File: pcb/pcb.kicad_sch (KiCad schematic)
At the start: 113 parts, among them J1 MJ-4PP-9, J2 MJ-4PP-9, J3 USB_C_Receptacle_USB2.0_16P, J4 USB to TTL, J5 Conn_01x03, J6 Conn_01x03, SW1 KEY_SW, SW10 KEY_SW, SW11 KEY_SW, SW12 KEY_SW, SW13 KEY_SW, SW14 KEY_SW, SW15 KEY_SW, SW16 KEY_SW, SW17 KEY_SW, SW18 KEY_SW, SW19 KEY_SW, SW2 KEY_SW, SW20 KEY_SW, SW21 KEY_SW, SW22 KEY_SW, SW23 KEY_SW, SW24 KEY_SW, SW25 KEY_SW, SW26 KEY_SW, SW27 RotaryEncoder, SW3 KEY_SW, SW30 KEY_SW, SW31 KEY_SW, SW32 KEY_SW, SW33 KEY_SW, SW34 KEY_SW, SW35 KEY_SW, SW36 KEY_SW, SW37 KEY_SW, SW38 KEY_SW, SW39 KEY_SW, SW4 KEY_SW, SW40 KEY_SW, SW41 KEY_SW, SW42 KEY_SW, SW43 KEY_SW, SW44 KEY_SW, SW45 KEY_SW, SW46 KEY_SW, SW47 KEY_SW, SW48 KEY_SW, SW49 KEY_SW, SW5 KEY_SW, SW50 KEY_SW, SW51 KEY_SW, SW52 KEY_SW, SW53 KEY_SW, SW54 KEY_SW, SW6 KEY_SW, SW60 RESET_SW, SW61 BOOT_SW, SW7 KEY_SW, SW8 KEY_SW, SW9 KEY_SW, SW６２1 DIP_SW, U1 ESP32-S3-WROOM-1, U2 TPS1117LV33S, U3 USBLC6-2SC6

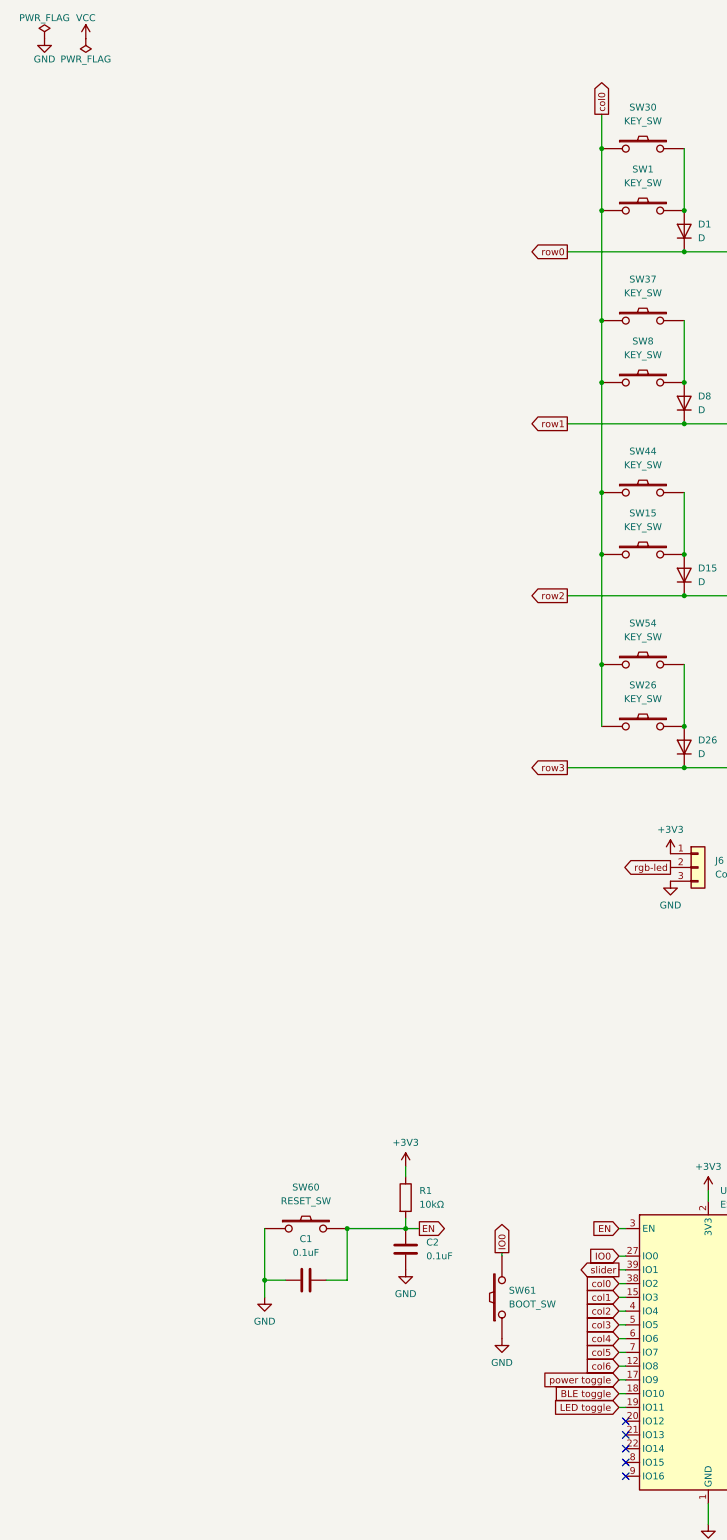
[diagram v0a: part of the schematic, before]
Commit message: connect
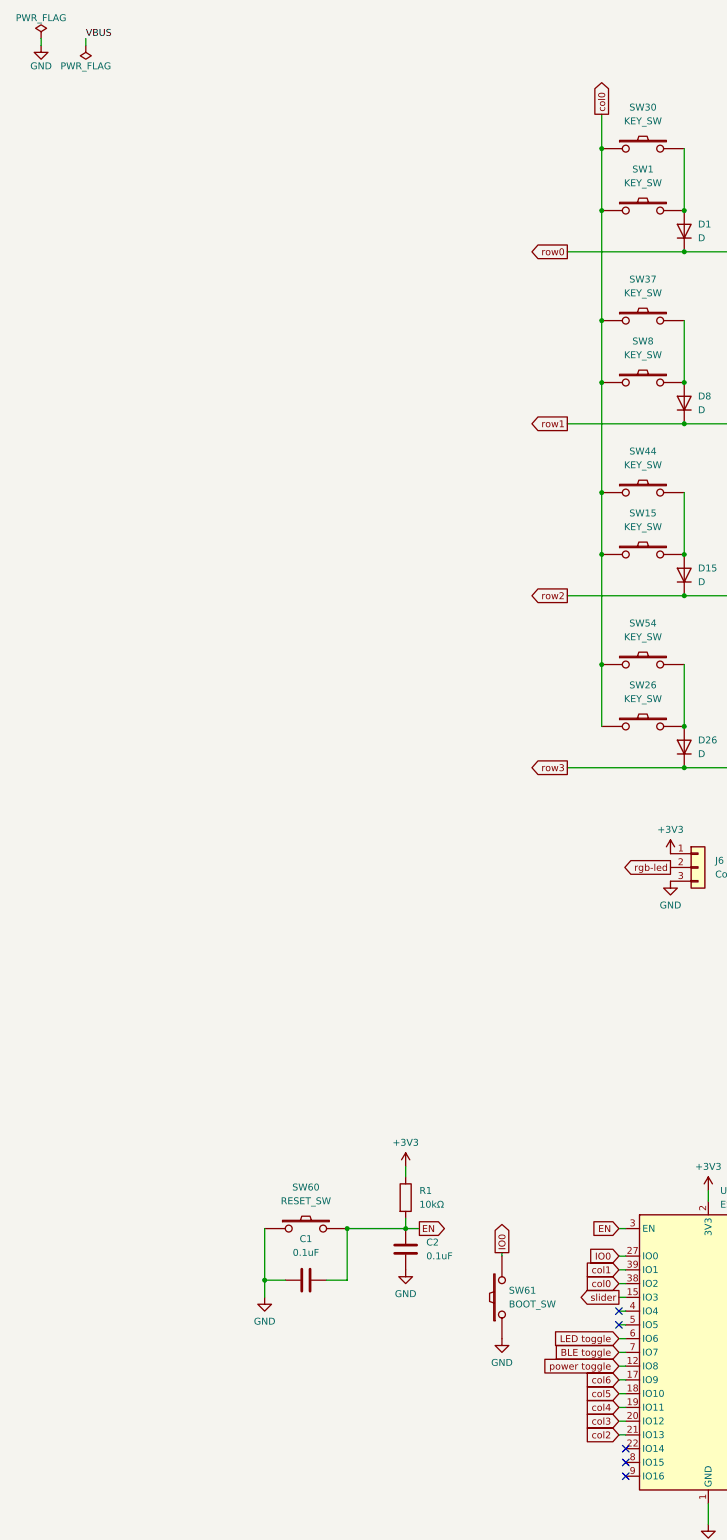
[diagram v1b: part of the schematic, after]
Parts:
- J3: footprint Connector_USB:USB_C_Receptacle_GCT_USB4105-xx-A_16P_TopMnt_Horizontal -> lib:USB_C_Receptacle_GCT_USB4105-xx-A_16P_TopMnt_Horizontal_rev
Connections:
- net BLE toggle: now also U1.7 (IO7); no longer U1.18 (IO10)
- net LED toggle: now also U1.6 (IO6); no longer U1.19 (IO11)
- net col1: now also U1.39 (IO1); no longer U1.15 (IO3)
- net col2: now also U1.21 (IO13); no longer U1.4 (IO4)
- net col3: now also U1.20 (IO12); no longer U1.5 (IO5)
- net col4: now also U1.19 (IO11); no longer U1.6 (IO6)
- net col5: now also U1.18 (IO10); no longer U1.7 (IO7)
- net col6: now also U1.17 (IO9); no longer U1.12 (IO8)
- net power toggle: now also U1.12 (IO8); no longer U1.17 (IO9)
- net slider: now also U1.15 (IO3); no longer U1.39 (IO1)
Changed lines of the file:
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@@
 	)
 	(no_connect
-		(at 142.875 240.03)
+		(at 111.125 242.57)
 	)
 	(no_connect
-		(at 112.395 260.35)
+		(at 142.875 240.03)
 	)
 	(no_connect
@@
 	)
 	(no_connect
-		(at 112.395 262.89)
+		(at 112.395 270.51)
 	)
 	(no_connect
-		(at 112.395 270.51)
+		(at 111.125 240.03)
 	)
 	(no_connect
@@
 	(wire
 		(pts
+			(xy 111.125 260.35) (xy 112.395 260.35)
+		)
+		(stroke
+			(width 0)
+			(type default)
+		)
+	)
+	(wire
+		(pts
 			(xy 254 186.055) (xy 254 187.325)
 		)
@@
 	(wire
 		(pts
+			(xy 12.7 6.35) (xy 12.7 5.08)
+		)
+		(stroke
+			(width 0)
+			(type default)
+		)
+	)
+	(wire
+		(pts
 			(xy 60.96 234.315) (xy 57.15 234.315)
 		)
@@
 	(wire
 		(pts
+			(xy 111.125 262.89) (xy 112.395 262.89)
+		)
+		(stroke
+			(width 0)
+			(type default)
+		)
+	)
+	(wire
+		(pts
 			(xy 233.68 149.225) (xy 233.68 150.495)
 		)
@@
 	(wire
 		(pts
+			(xy 4.445 6.35) (xy 4.445 5.08)
+		)
+		(stroke
+			(width 0)
+			(type default)
+		)
+	)
+	(wire
+		(pts
 			(xy 176.53 254) (xy 177.8 254)
 		)
@@
 		)
 	)
+	(label "VBUS"
+		(at 12.7 5.08 0)
+		(fields_autoplaced yes)
+		(effects
+			(font
+				(size 1.27 1.27)
+			)
+			(justify left bottom)
+		)
+	)
 	(global_label "col5"
 		(shape output)
@@
 	(global_label "LED toggle"
 		(shape input)
-		(at 111.125 257.81 180)
+		(at 111.125 245.11 180)
 		(fields_autoplaced yes)
 		(effects
@@
 		)
 		(property "Intersheetrefs" "${INTERSHEET_REFS}"
-			(at 97.7986 257.81 0)
+			(at 97.7986 245.11 0)
 			(effects
 				(font
@@
 	(global_label "col6"
 		(shape input)
-		(at 111.125 250.19 180)
+		(at 111.125 252.73 180)
 		(fields_autoplaced yes)
 		(effects
@@
 		)
 		(property "Intersheetrefs" "${INTERSHEET_REFS}"
-			(at 104.0275 250.19 0)
+			(at 104.0275 252.73 0)
 			(effects
 				(font
@@
 	(global_label "BLE toggle"
 		(shape input)
-		(at 111.125 255.27 180)
+		(at 111.125 247.65 180)
 		(fields_autoplaced yes)
 		(effects
@@
 		)
 		(property "Intersheetrefs" "${INTERSHEET_REFS}"
-			(at 97.7986 255.27 0)
+			(at 97.7986 247.65 0)
 			(effects
 				(font
@@
 	(global_label "power toggle"
 		(shape input)
-		(at 111.125 252.73 180)
+		(at 111.125 250.19 180)
 		(fields_autoplaced yes)
 		(effects
@@
 		)
 		(property "Intersheetrefs" "${INTERSHEET_REFS}"
-			(at 95.7424 252.73 0)
+			(at 95.7424 250.19 0)
 			(effects
 				(font
@@
 	(global_label "col2"
 		(shape input)
-		(at 111.125 240.03 180)
+		(at 111.125 262.89 180)
 		(fields_autoplaced yes)
 		(effects
@@
 		)
 		(property "Intersheetrefs" "${INTERSHEET_REFS}"
-			(at 104.0275 240.03 0)
+			(at 104.0275 262.89 0)
 			(effects
 				(font
@@
 	(global_label "col3"
 		(shape input)
-		(at 111.125 242.57 180)
+		(at 111.125 260.35 180)
 		(fields_autoplaced yes)
 		(effects
@@
 		)
 		(property "Intersheetrefs" "${INTERSHEET_REFS}"
-			(at 104.0275 242.57 0)
+			(at 104.0275 260.35 0)
 			(effects
 				(font
@@
 	(global_label "col5"
 		(shape input)
-		(at 111.125 247.65 180)
+		(at 111.125 255.27 180)
 		(fields_autoplaced yes)
 		(effects
@@
 		)
 		(property "Intersheetrefs" "${INTERSHEET_REFS}"
-			(at 104.0275 247.65 0)
+			(at 104.0275 255.27 0)
 			(effects
 				(font
@@
 	(global_label "col1"
 		(shape input)
-		(at 111.125 237.49 180)
+		(at 111.125 232.41 180)
 		(fields_autoplaced yes)
 		(effects
@@
 		)
 		(property "Intersheetrefs" "${INTERSHEET_REFS}"
-			(at 104.0275 237.49 0)
+			(at 104.0275 232.41 0)
 			(effects
 				(font
@@
 	(global_label "col4"
 		(shape input)
-		(at 111.125 245.11 180)
+		(at 111.125 257.81 180)
 		(fields_autoplaced yes)
 		(effects
@@
 		)
 		(property "Intersheetrefs" "${INTERSHEET_REFS}"
-			(at 104.0275 245.11 0)
+			(at 104.0275 257.81 0)
 			(effects
 				(font
@@
 	(global_label "slider"
 		(shape output)
-		(at 111.125 232.41 180)
+		(at 111.125 237.49 180)
 		(fields_autoplaced yes)
 		(effects
@@
 		)
 		(property "Intersheetrefs" "${INTERSHEET_REFS}"
-			(at 102.8179 232.41 0)
+			(at 102.8179 237.49 0)
 			(effects
 				(font
@@
 	)
 	(symbol
-		(lib_id "power:VCC")
-		(at 12.7 5.08 0)
-		(unit 1)
-		(exclude_from_sim no)
-		(in_bom yes)
-		(on_board yes)
-		(dnp no)
-		(property "Reference" "#PWR05"
-			(at 12.7 8.89 0)
-			(effects
-				(font
-					(size 1.27 1.27)
-				)
-				(hide yes)
-			)
-		)
-		(property "Value" "VCC"
-			(at 12.7 1.27 0)
-			(effects
-				(font
-					(size 1.27 1.27)
-				)
-			)
-		)
-		(property "Footprint" ""
-			(at 12.7 5.08 0)
-			(effects
-				(font
-					(size 1.27 1.27)
-				)
-				(hide yes)
-			)
-		)
-		(property "Datasheet" ""
-			(at 12.7 5.08 0)
-			(effects
-				(font
-					(size 1.27 1.27)
-				)
-				(hide yes)
-			)
-		)
-		(property "Description" ""
-			(at 12.7 5.08 0)
-			(effects
-				(font
-					(size 1.27 1.27)
-				)
-				(hide yes)
-			)
-		)
-		(pin "1"
-		)
-		(instances
-			(project "pcb"
-				(path "/ca1682eb-af97-4baf-a70b-d30c3b256c66"
-					(reference "#PWR05")
-					(unit 1)
-				)
-			)
-		)
-	)
-	(symbol
 		(lib_id "Device:D")
 		(at 173.99 104.14 90)
@@
 			)
 		)
-		(property "Footprint" "Connector_USB:USB_C_Receptacle_GCT_USB4105-xx-A_16P_TopMnt_Horizontal"
+		(property "Footprint" "lib:USB_C_Receptacle_GCT_USB4105-xx-A_16P_TopMnt_Horizontal_rev"
 			(at 207.645 234.95 0)
 			(effects
@@
 	(symbol
 		(lib_id "power:PWR_FLAG")
-		(at 5.08 5.08 0)
+		(at 4.445 5.08 0)
 		(unit 1)
 		(exclude_from_sim no)
@@
 		(dnp no)
 		(property "Reference" "#FLG01"
-			(at 5.08 3.175 0)
+			(at 4.445 3.175 0)
 			(effects
 				(font
@@
 		)
 		(property "Value" "PWR_FLAG"
-			(at 5.08 1.27 0)
+			(at 4.445 1.27 0)
 			(effects
 				(font
@@
 		)
 		(property "Footprint" ""
-			(at 5.08 5.08 0)
+			(at 4.445 5.08 0)
 			(effects
 				(font
@@
 		)
 		(property "Datasheet" "~"
-			(at 5.08 5.08 0)
+			(at 4.445 5.08 0)
 			(effects
 				(font
@@
 		)
 		(property "Description" ""
-			(at 5.08 5.08 0)
+			(at 4.445 5.08 0)
 			(effects
 				(font
@@
 	(symbol
 		(lib_id "power:GND")
-		(at 5.08 5.08 0)
+		(at 4.445 6.35 0)
 		(unit 1)
 		(exclude_from_sim no)
@@
 		(dnp no)
 		(property "Reference" "#PWR04"
-			(at 5.08 11.43 0)
+			(at 4.445 12.7 0)
 			(effects
 				(font
@@
 		)
 		(property "Value" "GND"
-			(at 5.08 8.89 0)
+			(at 4.445 10.16 0)
 			(effects
 				(font
@@
 		)
 		(property "Footprint" ""
-			(at 5.08 5.08 0)
+			(at 4.445 6.35 0)
 			(effects
 				(font
@@
 		)
 		(property "Datasheet" ""
-			(at 5.08 5.08 0)
+			(at 4.445 6.35 0)
 			(effects
 				(font
@@
 		)
 		(property "Description" ""
-			(at 5.08 5.08 0)
+			(at 4.445 6.35 0)
 			(effects
 				(font
@@
 	(symbol
 		(lib_id "power:PWR_FLAG")
-		(at 12.7 5.08 180)
+		(at 12.7 6.35 180)
 		(unit 1)
 		(exclude_from_sim no)
@@
 		(dnp no)
 		(property "Reference" "#FLG02"
-			(at 12.7 6.985 0)
+			(at 12.7 8.255 0)
 			(effects
 				(font
@@
 		)
 		(property "Value" "PWR_FLAG"
-			(at 12.7 8.89 0)
+			(at 12.7 10.16 0)
 			(effects
 				(font
@@
 		)
 		(property "Footprint" ""
-			(at 12.7 5.08 0)
+			(at 12.7 6.35 0)
 			(effects
 				(font
@@
 		)
 		(property "Datasheet" "~"
-			(at 12.7 5.08 0)
+			(at 12.7 6.35 0)
 			(effects
 				(font
@@
 		)
 		(property "Description" ""
-			(at 12.7 5.08 0)
+			(at 12.7 6.35 0)
 			(effects
 				(font
